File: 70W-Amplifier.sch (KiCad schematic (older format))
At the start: 35 parts, among them J1 RF_OUT, J2 RF_IN, J3 LPF_IN, J4 LPF_OUT, J5 13.8V Input, J6 PTT, K1 G5V-2, Q1 2N3906-SMD, Q2 IRF530, Q3 IRF530, T1 BN-43-202 1T:2T, T2 Ferrite 1T:3T, U1 L7805

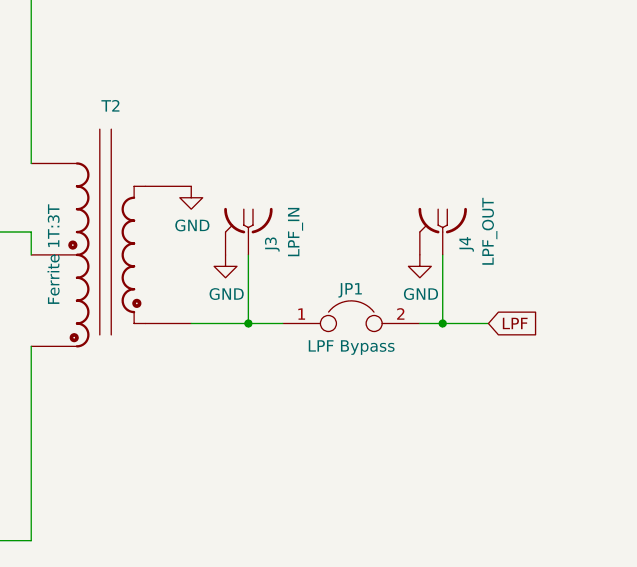
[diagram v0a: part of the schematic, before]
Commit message: added dc block cap
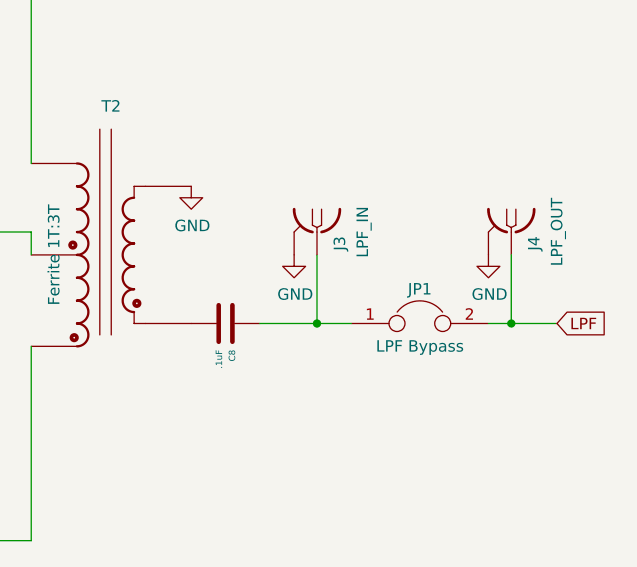
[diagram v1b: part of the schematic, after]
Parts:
- added C8: .1uF, Xenir:Capacitor 1206, symbol Xenir:Capacitor
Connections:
- net at J3.1, JP1.1: now also C8.1; no longer T2.1
- new net: C8.2, T2.1
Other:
- moved on the sheet: J3, J4, JP1
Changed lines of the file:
@@
 L power:GND #PWR019
 U 1 1 61D35B7D
-P 9050 4450
-F 0 "#PWR019" H 9050 4200 50  0001 C CNN
-F 1 "GND" H 9055 4277 50  0000 C CNN
-F 2 "" H 9050 4450 50  0001 C CNN
-F 3 "" H 9050 4450 50  0001 C CNN
-	1    9050 4450
+P 9350 4450
+F 0 "#PWR019" H 9350 4200 50  0001 C CNN
+F 1 "GND" H 9355 4277 50  0000 C CNN
+F 2 "" H 9350 4450 50  0001 C CNN
+F 3 "" H 9350 4450 50  0001 C CNN
+	1    9350 4450
 	1    0    0    -1
 $EndComp
@@
 L power:GND #PWR020
 U 1 1 61D35F33
-P 9900 4450
-F 0 "#PWR020" H 9900 4200 50  0001 C CNN
-F 1 "GND" H 9905 4277 50  0000 C CNN
-F 2 "" H 9900 4450 50  0001 C CNN
-F 3 "" H 9900 4450 50  0001 C CNN
-	1    9900 4450
-	1    0    0    -1
-$EndComp
-Wire Wire Line
-	9150 4450 9150 4750
-Wire Wire Line
-	9150 4750 8900 4750
-Text GLabel 10200 4750 2    50   Input ~ 0
+P 10200 4450
+F 0 "#PWR020" H 10200 4200 50  0001 C CNN
+F 1 "GND" H 10205 4277 50  0000 C CNN
+F 2 "" H 10200 4450 50  0001 C CNN
+F 3 "" H 10200 4450 50  0001 C CNN
+	1    10200 4450
+	1    0    0    -1
+$EndComp
+Wire Wire Line
+	9450 4450 9450 4750
+Wire Wire Line
+	9450 4750 9200 4750
+Text GLabel 10500 4750 2    50   Input ~ 0
 LPF
 Wire Wire Line
-	10000 4450 10000 4750
-Wire Wire Line
-	10000 4750 10200 4750
+	10300 4450 10300 4750
+Wire Wire Line
+	10300 4750 10500 4750
 $Comp
 L Device:Jumper JP1
 U 1 1 61D3D93E
-P 9600 4750
-F 0 "JP1" H 9600 4900 50  0000 C CNN
-F 1 "LPF Bypass" H 9600 4650 50  0000 C CNN
-F 2 "Xenir:Jumper" H 9600 4750 50  0001 C CNN
-F 3 "~" H 9600 4750 50  0001 C CNN
-	1    9600 4750
-	1    0    0    -1
-$EndComp
-Wire Wire Line
-	9900 4750 10000 4750
-Connection ~ 10000 4750
-Wire Wire Line
-	9300 4750 9150 4750
-Connection ~ 9150 4750
+P 9900 4750
+F 0 "JP1" H 9900 4900 50  0000 C CNN
+F 1 "LPF Bypass" H 9900 4650 50  0000 C CNN
+F 2 "Xenir:Jumper" H 9900 4750 50  0001 C CNN
+F 3 "~" H 9900 4750 50  0001 C CNN
+	1    9900 4750
+	1    0    0    -1
+$EndComp
+Wire Wire Line
+	10200 4750 10300 4750
+Connection ~ 10300 4750
+Wire Wire Line
+	9600 4750 9450 4750
+Connection ~ 9450 4750
 Wire Wire Line
 	6050 4350 6050 4250
@@
 L Xenir:PCB_SMA_EDGE J3
 U 1 1 61CF5952
-P 9350 4350
-F 0 "J3" H 9400 4250 50  0000 C CNN
-F 1 "LPF_IN" H 9350 4350 50  0000 C CNN
-F 2 "Xenir:PCB-SMA-EDGE" H 9350 4350 50  0001 C CNN
-F 3 "" H 9350 4350 50  0001 C CNN
-	1    9350 4350
+P 9650 4350
+F 0 "J3" H 9700 4250 50  0000 C CNN
+F 1 "LPF_IN" H 9650 4350 50  0000 C CNN
+F 2 "Xenir:PCB-SMA-EDGE" H 9650 4350 50  0001 C CNN
+F 3 "" H 9650 4350 50  0001 C CNN
+	1    9650 4350
 	0    1    1    0
 $EndComp
@@
 L Xenir:PCB_SMA_EDGE J4
 U 1 1 61CF9C6B
-P 10200 4350
-F 0 "J4" H 10250 4250 50  0000 C CNN
-F 1 "LPF_OUT" H 10200 4350 50  0000 C CNN
-F 2 "Xenir:PCB-SMA-EDGE" H 10200 4350 50  0001 C CNN
-F 3 "" H 10200 4350 50  0001 C CNN
-	1    10200 4350
+P 10500 4350
+F 0 "J4" H 10550 4250 50  0000 C CNN
+F 1 "LPF_OUT" H 10500 4350 50  0000 C CNN
+F 2 "Xenir:PCB-SMA-EDGE" H 10500 4350 50  0001 C CNN
+F 3 "" H 10500 4350 50  0001 C CNN
+	1    10500 4350
 	0    1    1    0
 $EndComp
@@
 Wire Wire Line
 	7350 4550 7350 4450
+$Comp
+L Xenir:Capacitor C8
+U 1 1 61E9AE04
+P 9050 4750
+F 0 "C8" V 9021 4865 28  0000 L CNN
+F 1 ".1uF" V 9078 4865 28  0000 L CNN
+F 2 "Xenir:Capacitor 1206" H 9050 4600 50  0001 C CNN
+F 3 "" H 9050 4600 50  0001 C CNN
+	1    9050 4750
+	-1   0    0    1
+$EndComp
 $EndSCHEMATC
